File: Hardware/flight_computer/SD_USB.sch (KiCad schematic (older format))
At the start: 30 parts

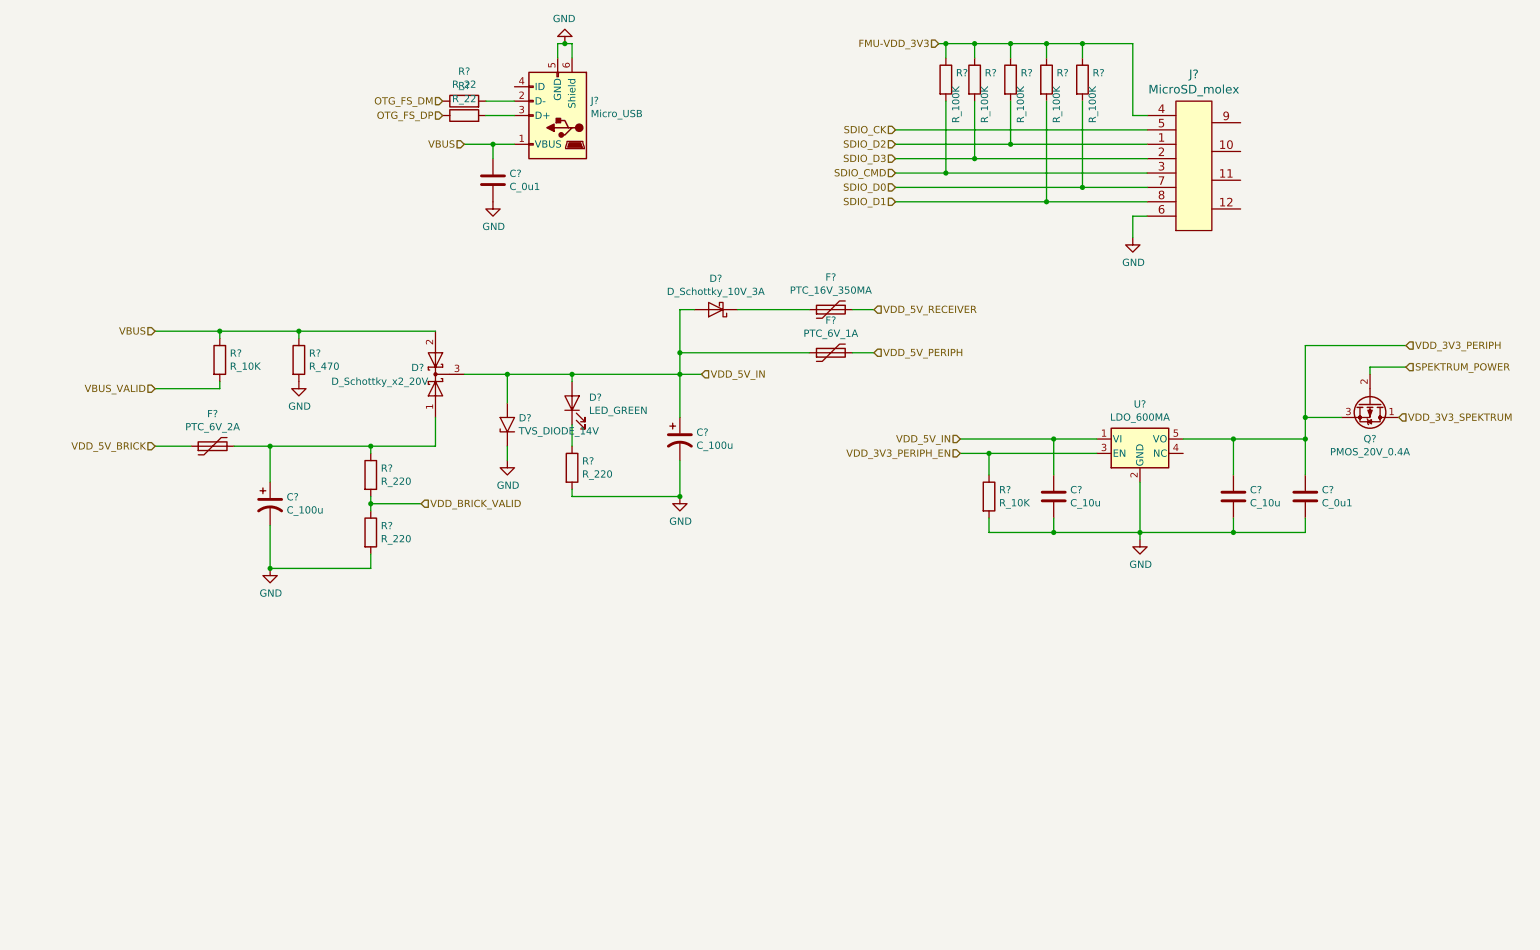
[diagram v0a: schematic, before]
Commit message: added components, rerranged things to slow down dan
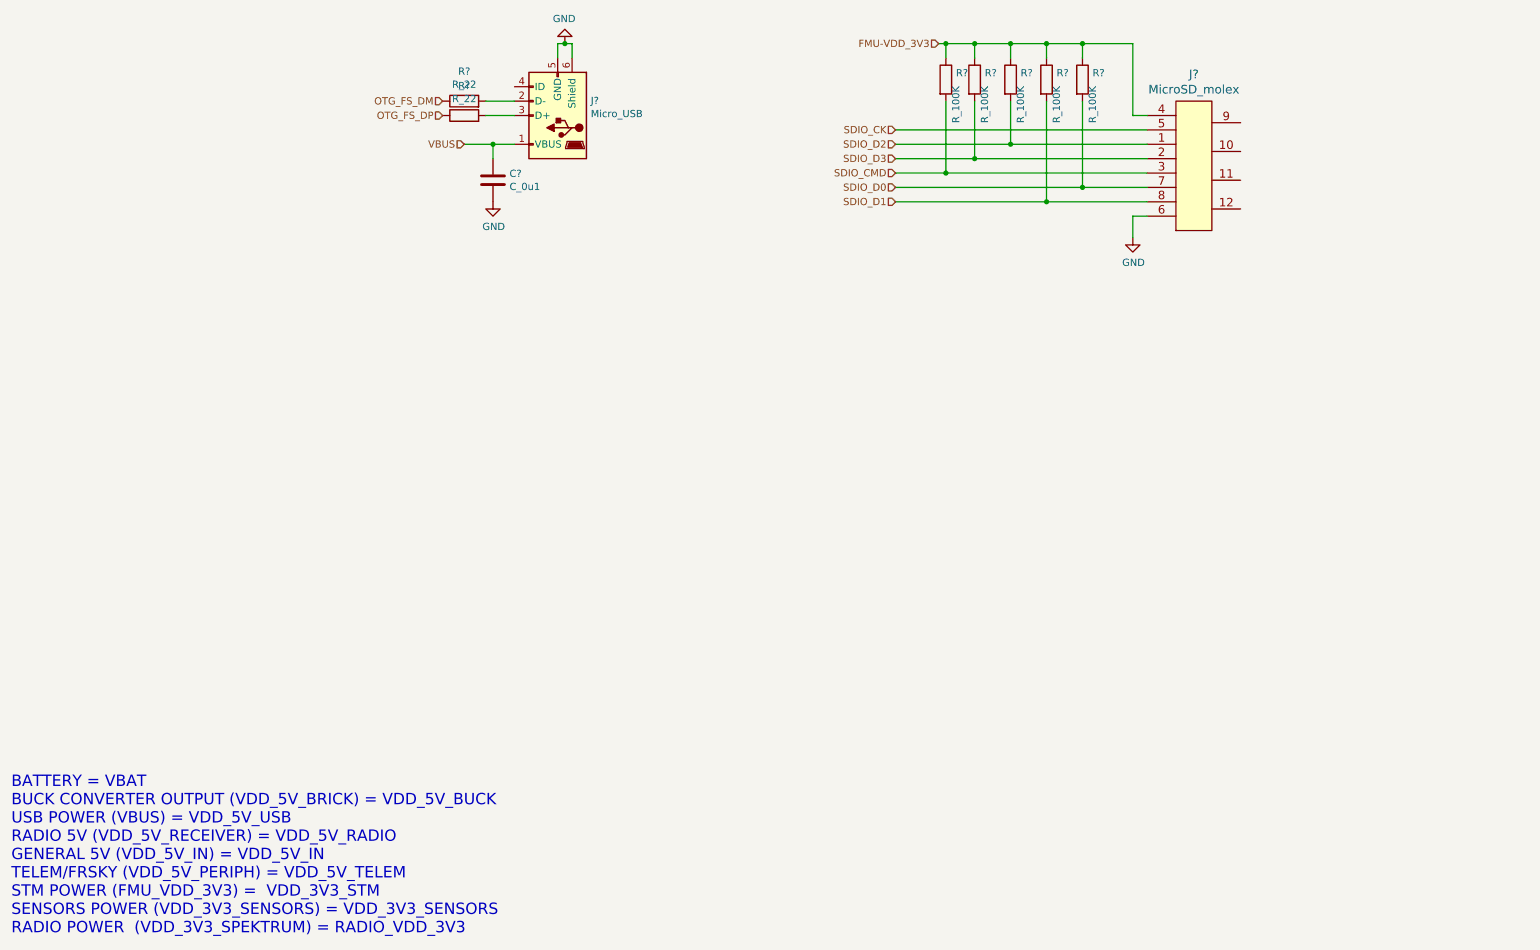
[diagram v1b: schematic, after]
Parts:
- removed C? (x2): C_100u, drone_footprints:10SGV100M6.3X6.1, symbol openDrone_parts:C_100u
- removed C? (x2): C_10u, Capacitors_SMD:C_0805, symbol openDrone_parts:C_10u
- removed C?: C_0u1, Capacitors_SMD:C_0805, symbol openDrone_parts:C_0u1
- removed D?: D_Schottky_x2_20V, drone_footprints:SOT1061, symbol openDrone_parts:D_Schottky_x2_20V
- removed D?: LED_GREEN, LEDs:LED_0603_HandSoldering, symbol openDrone_parts:LED_GREEN
- removed D?: D_Schottky_10V_3A, Diodes_SMD:D_SOD-323F, symbol openDrone_parts:D_Schottky_10V_3A
- removed D?: TVS_DIODE_14V, Capacitors_SMD:C_0402, symbol openDrone_parts:TVS_DIODE_14V
- removed F?: PTC_6V_2A, Fuse_Holders_and_Fuses:Fuse_SMD1206_HandSoldering, symbol openDrone_parts:PTC_6V_2A
- removed F?: PTC_16V_350MA, Resistors_SMD:R_0805_HandSoldering, symbol openDrone_parts:PTC_16V_350MA
- removed F?: PTC_6V_1A, Resistors_SMD:R_0805_HandSoldering, symbol openDrone_parts:PTC_6V_1A
- removed Q?: PMOS_20V_0.4A, TO_SOT_Packages_SMD:SOT-323_SC-70, symbol openDrone_parts:PMOS_20V_0.4A
- removed R? (x2): R_10K, Resistors_SMD:R_0805, symbol openDrone_parts:R_10K
- removed R? (x3): R_220, Resistors_SMD:R_0805, symbol openDrone_parts:R_220
- removed R?: R_470, Resistors_SMD:R_0805, symbol openDrone_parts:R_470
- removed U?: LDO_600MA, drone_footprints:SOT-25_DIO, symbol openDrone_parts:LDO_600MA
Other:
- note added: "BATTERY = VBAT\nBUCK CONVERTER OUTPUT (VDD_5V_BRICK) = VDD_5V_BUCK\nUSB POWER (VBUS) = VDD_5V_USB\nRADIO 5V (VDD_5V_RECEIVER) = VDD_5V_RADIO\nGENERAL 5V (VDD_5V_IN) = VDD_5V_IN\nTELEM/FRSKY (VDD_5V_PERIPH) = VDD_5V_TELEM\nSTM POWER (FMU_VDD_3V3) = VDD_3V3_STM\nSENSORS POWER (VDD_3V3_SENSORS) = VDD_3V3_SENSORS\nRADIO POWER (VDD_3V3_SPEKTRUM) = RADIO_VDD_3V3\n"
